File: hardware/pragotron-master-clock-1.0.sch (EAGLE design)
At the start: 65 parts, among them IC1 ATSAMD21E18A-MU, IC2 AP2112K-3.3, IC3 MIC2288YD5-TR, IC4 DS3231MZ+, J1 USB-C, J2 TRMBLK_3.5MM_2P, J3 2X5_PITCH_1.27MMTH_NOKEY_UNSH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, Q1 N-MOSFET, Q2 N-MOSFET, Q3 N-MOSFET, Q4 N-MOSFET, Q5 P-MOSFET, Q6 P-MOSFET

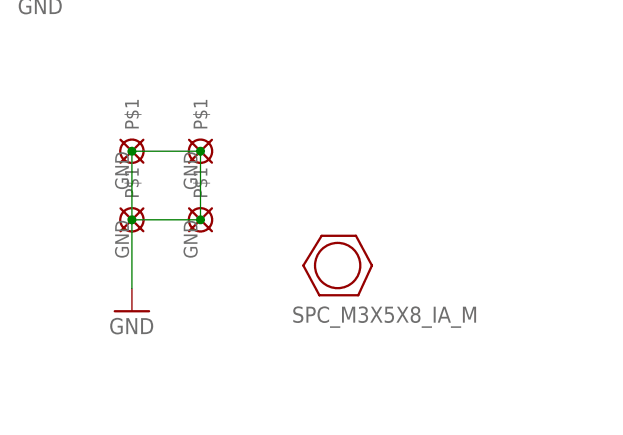
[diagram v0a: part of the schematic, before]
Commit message: small fixes
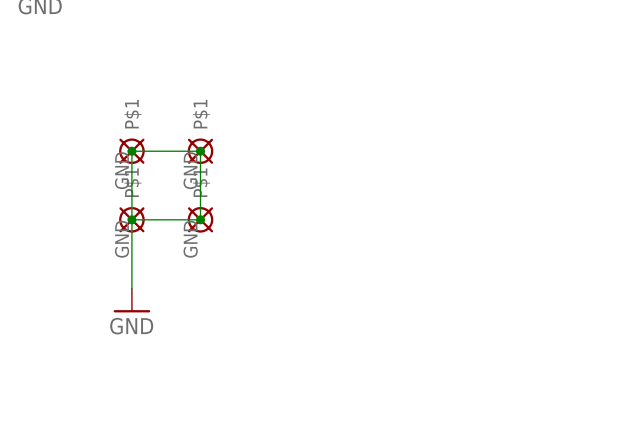
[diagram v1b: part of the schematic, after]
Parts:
- removed HW1: SPC_M3X5X8_IA_M, BASTL_MECHANICAL:SPC_M3X5X8_IA_M
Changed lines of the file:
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@@
 <part name="SUPPLY6" library="BASTL_SYMBOLS" library_urn="urn:adsk.eagle:library:32975873" deviceset="VDD" device=""/>
 <part name="SUPPLY5" library="BASTL_SYMBOLS" library_urn="urn:adsk.eagle:library:32975873" deviceset="VDD" device=""/>
-<part name="HW1" library="BASTL_MECHANICAL" library_urn="urn:adsk.eagle:library:32977656" deviceset="SPC_M3X5X8_IA_M" device="" package3d_urn="urn:adsk.eagle:package:42477236/2"/>
 </parts>
 <sheets>
@@
 <attribute name="VALUE" x="241.935" y="-103.505" size="1.778" layer="96"/>
 </instance>
-<instance part="HW1" gate="G$1" x="309.88" y="-109.22" smashed="yes">
-<attribute name="VALUE" x="304.8" y="-115.57" size="1.778" layer="96"/>
-</instance>
 </instances>

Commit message: small fixes
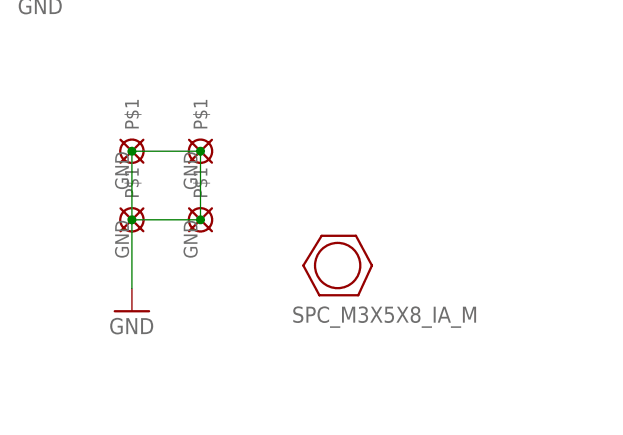
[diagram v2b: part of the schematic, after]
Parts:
- added HW1: SPC_M3X5X8_IA_M, BASTL_MECHANICAL:SPC_M3X5X8_IA_M
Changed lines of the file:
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@@
 <part name="SUPPLY6" library="BASTL_SYMBOLS" library_urn="urn:adsk.eagle:library:32975873" deviceset="VDD" device=""/>
 <part name="SUPPLY5" library="BASTL_SYMBOLS" library_urn="urn:adsk.eagle:library:32975873" deviceset="VDD" device=""/>
+<part name="HW1" library="BASTL_MECHANICAL" library_urn="urn:adsk.eagle:library:32977656" deviceset="SPC_M3X5X8_IA_M" device="" package3d_urn="urn:adsk.eagle:package:42477236/2"/>
 </parts>
 <sheets>
@@
 <attribute name="VALUE" x="241.935" y="-103.505" size="1.778" layer="96"/>
 </instance>
+<instance part="HW1" gate="G$1" x="309.88" y="-109.22" smashed="yes">
+<attribute name="VALUE" x="304.8" y="-115.57" size="1.778" layer="96"/>
+</instance>
 </instances>
